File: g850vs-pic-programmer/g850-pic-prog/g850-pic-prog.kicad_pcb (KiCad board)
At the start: 2 copper layers, 106.7 x 36.1 mm, 30 parts, among them J1 Conn_01x11_Male, Q1 BC547, Q2 2N3906, Q3 BC547, U1 74HC14, U2 PIC16F84-XXP

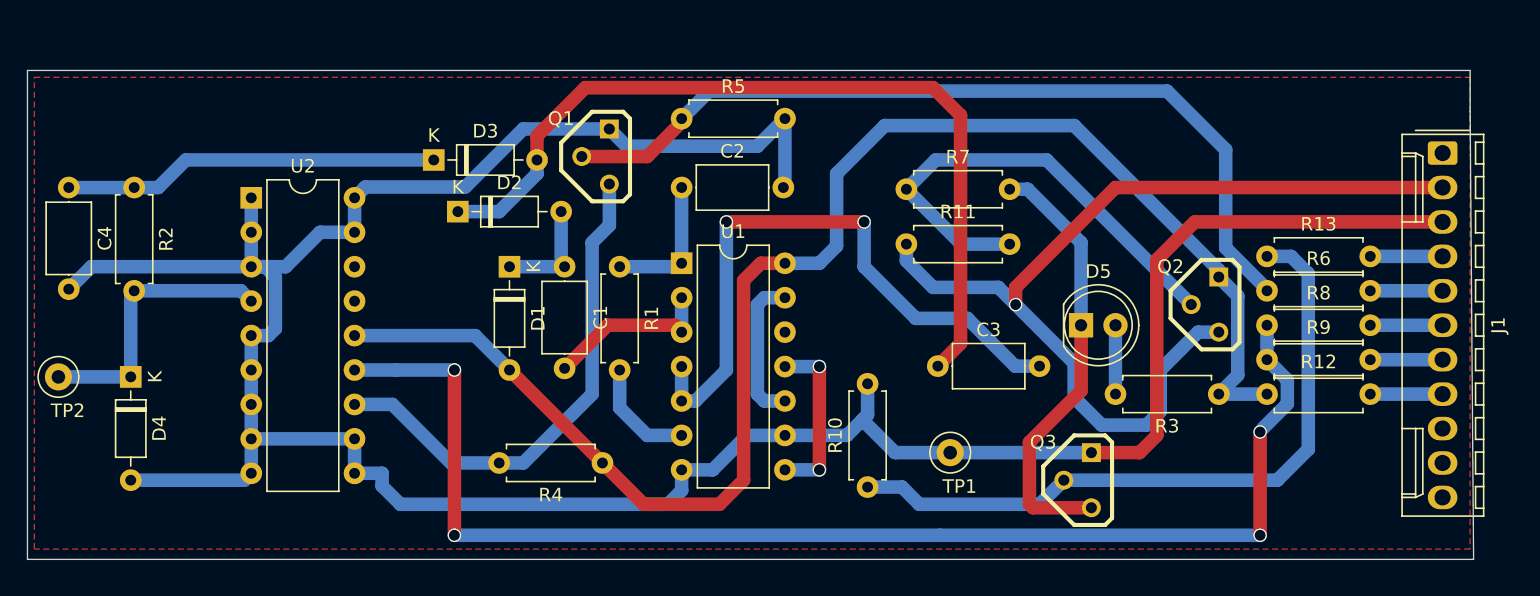
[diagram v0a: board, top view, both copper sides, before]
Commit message: Updates
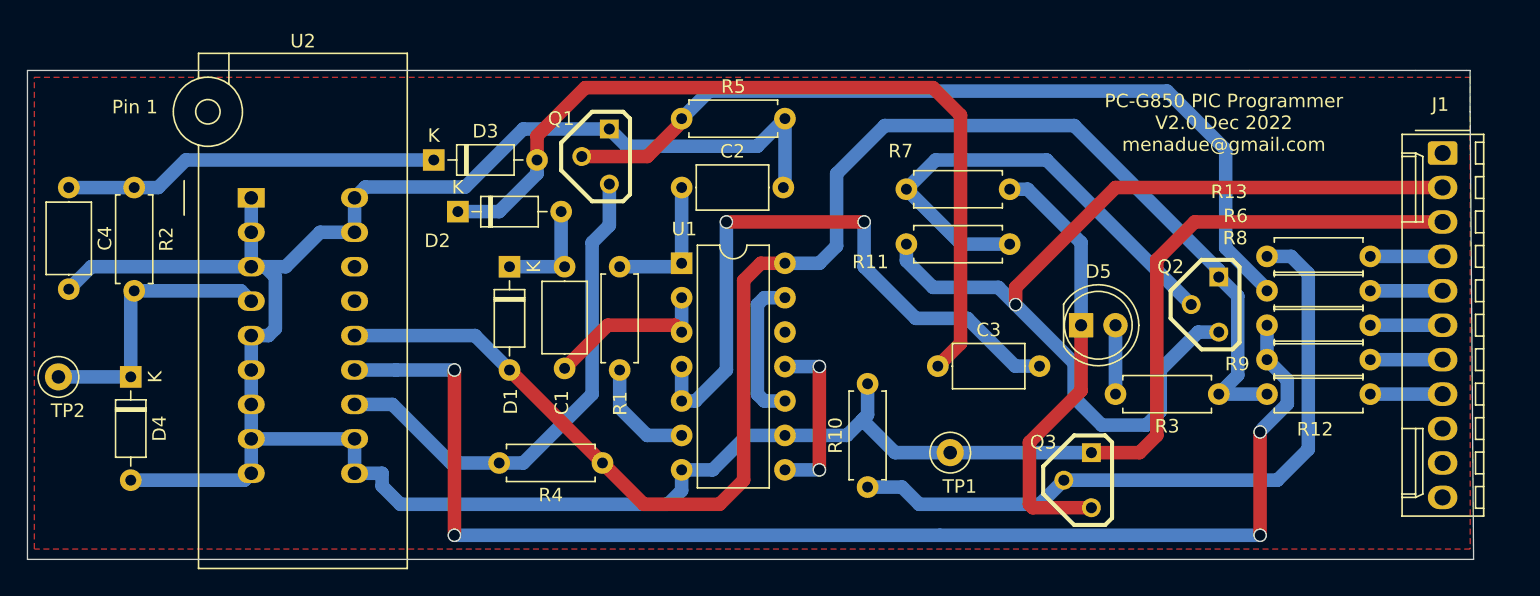
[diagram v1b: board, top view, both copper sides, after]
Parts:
- C1, C3, C4: value 680pF -> 10nF
- C2: value 680pF -> n27
- U2: footprint Package_DIP:DIP-18_W7.62mm -> Socket:DIP_Socket-18_W4.3_W5.08_W7.62_W10.16_W10.9_3M_218-3341-00-0602J
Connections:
- J1 pad 1: Net-(J1-Pad1) -> (no net)
- J1 pad 10: Net-(J1-Pad10) -> (no net)
- J1 pad 11: Net-(J1-Pad11) -> (no net)
- J1 pad 9: Net-(J1-Pad9) -> (no net)
- U1 pad 12: Net-(U1-Pad12) -> (no net)
- U2 pad 15: Net-(U2-Pad15) -> (no net)
- U2 pad 16: Net-(U2-Pad16) -> (no net)
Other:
- board text added: "PC-G850 PIC Programmer V2.0 Dec 2022 menadue@gmail.com"
- board text added: "Pin 1"
